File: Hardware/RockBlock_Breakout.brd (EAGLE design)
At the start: 25.4 x 53 mm, 24 parts, among them J1 CONN_62.54, J2 CONN_82.54, U1 ATMEGA328P_TQFP, U4 TPS61027DRC, Y1 16MHz

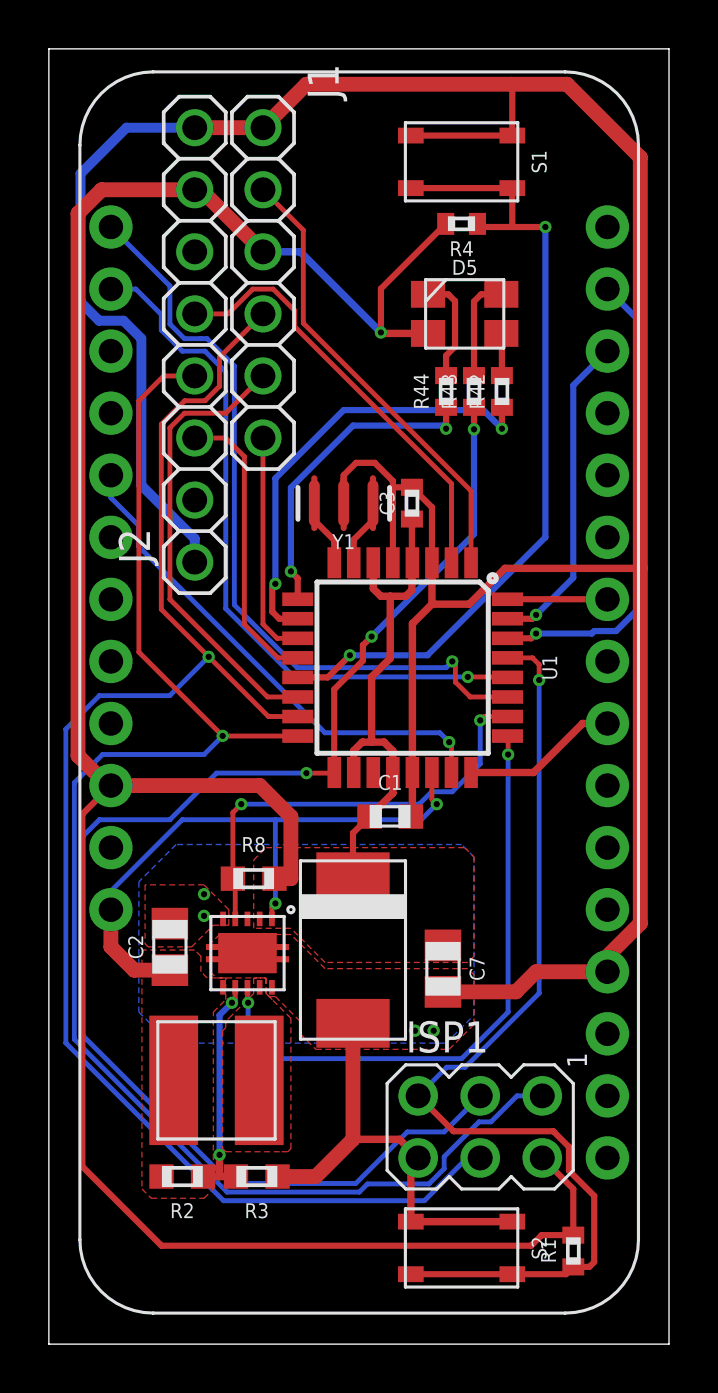
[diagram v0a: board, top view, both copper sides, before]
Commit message: Routing cleanup
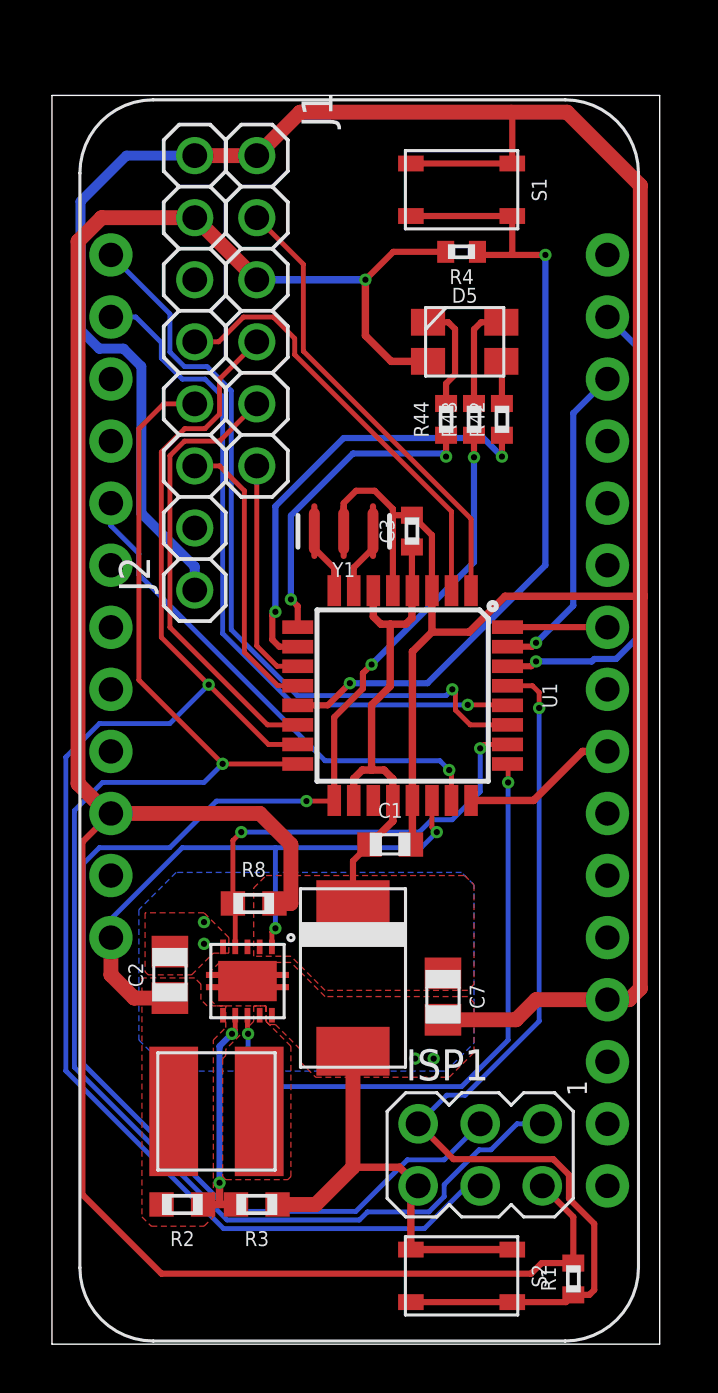
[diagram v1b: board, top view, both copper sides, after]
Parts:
- moved L2 1.27 mm to (6.86, 9.53)
- moved J1 1.17 mm to (8.51, 42.3)
- moved C1 1.14 mm to (14.0, 20.4)
- moved C2 1.14 mm to (4.95, 15.1)
- moved C3 1.14 mm to (14.9, 33.3)
- moved C5 1.14 mm to (12.4, 15.0)
- moved C7 1.14 mm to (16.1, 14.2)
- moved D5 1.14 mm to (17.0, 41.0)
- moved ISP1 1.14 mm to (17.7, 7.75)
- moved J2 1.14 mm to (5.97, 39.8)
- moved R4 1.14 mm to (16.9, 44.7)
- moved R42 1.14 mm to (18.5, 37.8)
- moved R43 1.14 mm to (17.4, 37.8)
- moved R44 1.14 mm to (16.3, 37.8)
- moved S1 1.14 mm to (16.9, 47.2)
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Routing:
- net 5V: track 119.9 -> 119.4 mm
- net GND: track 140.8 -> 141.3 mm
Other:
- board size 25.4 x 53 mm -> 24.9 x 51.1 mm
